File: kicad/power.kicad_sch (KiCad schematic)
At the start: 19 parts, among them J25 ATX-24, J26 External Power, SW2 POWER ON

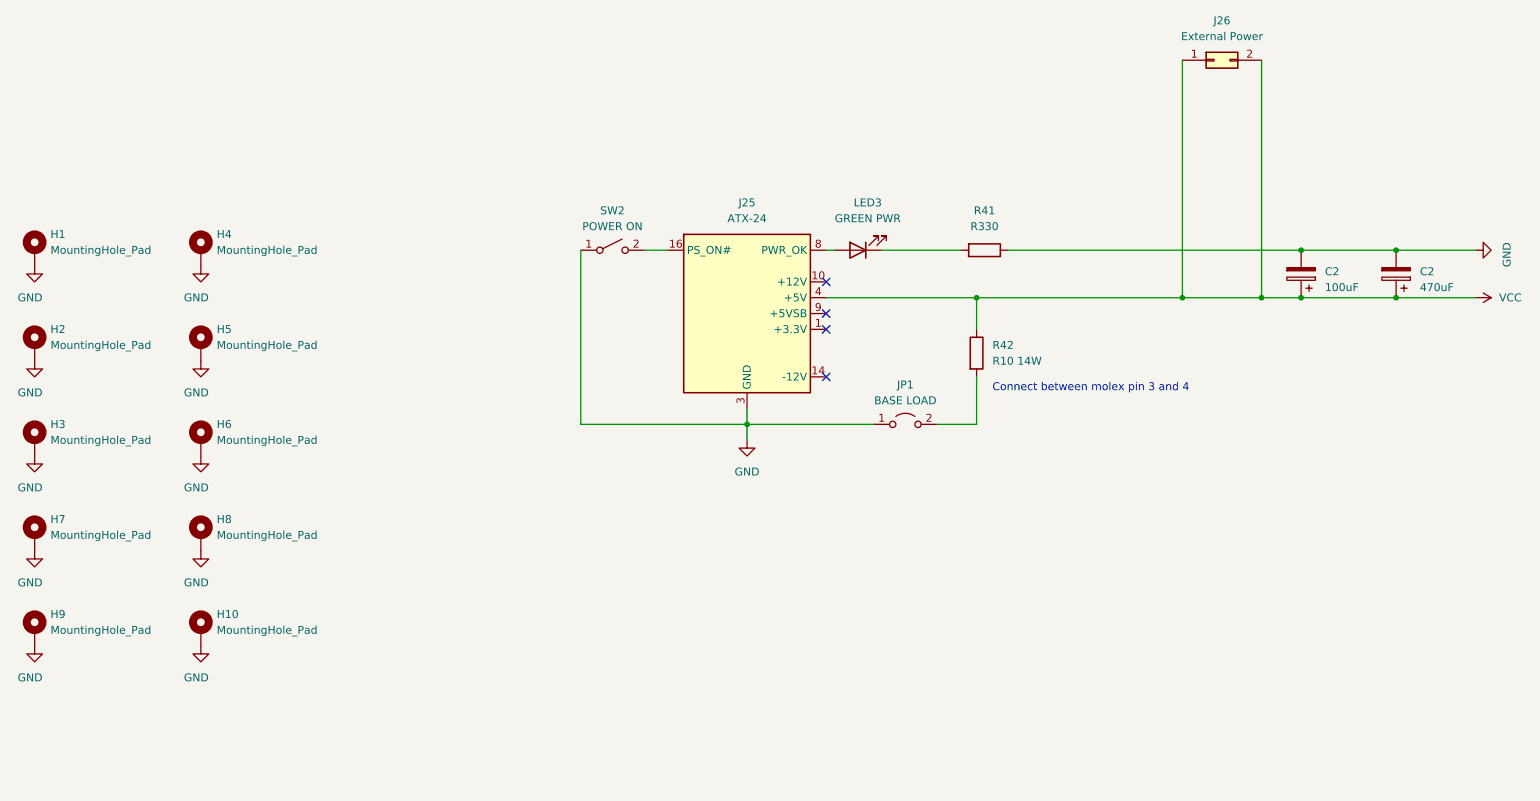
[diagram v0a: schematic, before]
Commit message: fiddlign with placement
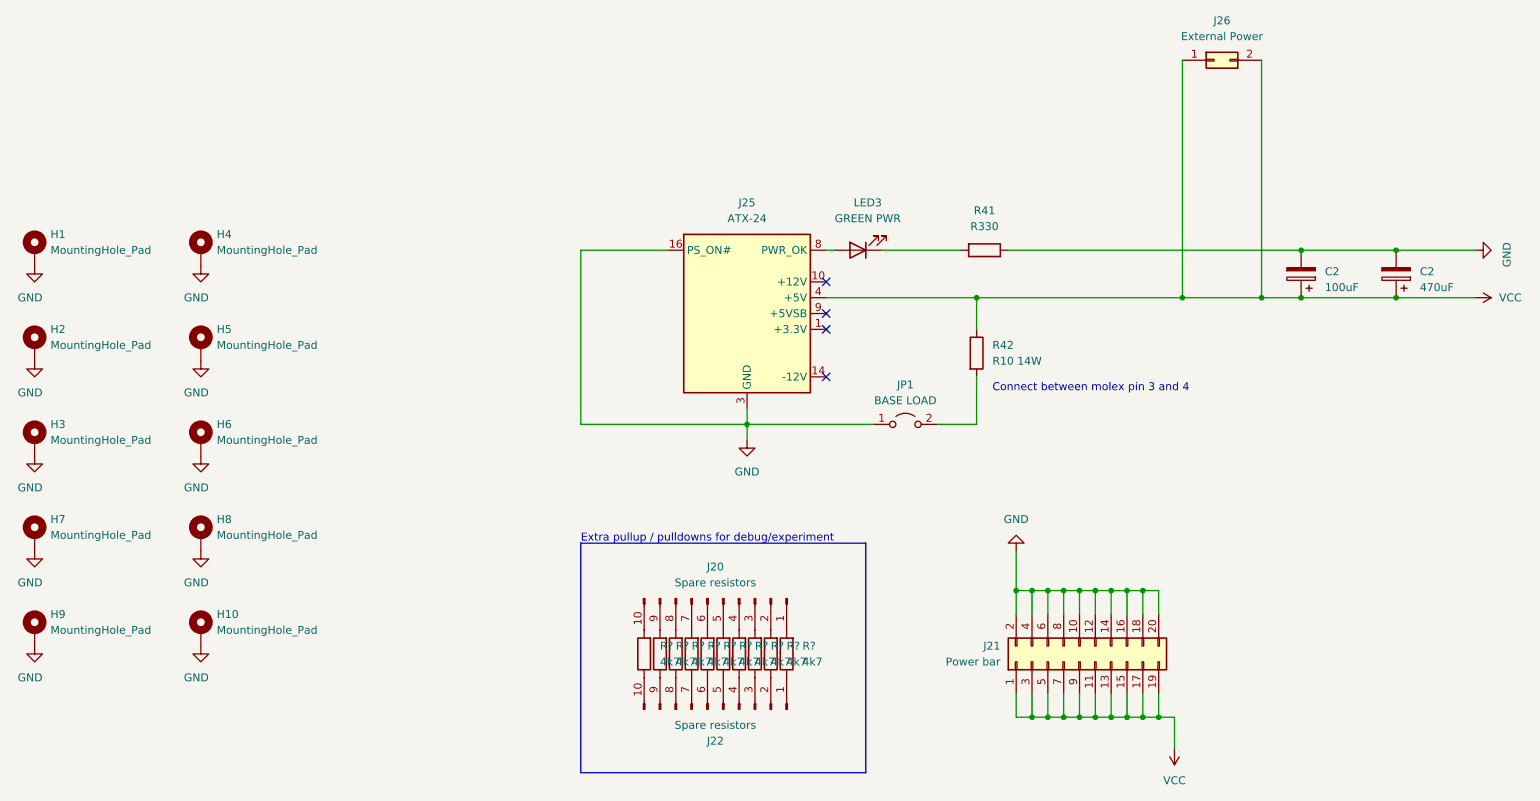
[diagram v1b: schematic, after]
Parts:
- removed SW2: POWER ON, Button_Switch_SMD:SW_DIP_SPSTx01_Slide_6.7x4.1mm_W8.61mm_P2.54mm_LowProfile, symbol Switch:SW_SPST
- added J20, J22: Spare resistors, Connector_PinSocket_2.54mm:PinSocket_1x10_P2.54mm_Vertical, symbol Connector:Conn_01x10_Pin
- added J21: Power bar, Connector_PinSocket_2.54mm:PinSocket_2x10_P2.54mm_Vertical, symbol Connector_Generic:Conn_02x10_Odd_Even
- added R? (x10): 4k7, Resistor_THT:R_Axial_DIN0207_L6.3mm_D2.5mm_P10.16mm_Horizontal, symbol Device:R
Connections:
- net GND: now also J25.16 (PS_ON#), J21.10 (Pin_10), J21.12 (Pin_12), J21.14 (Pin_14), J21.16 (Pin_16), J21.18 (Pin_18), J21.2 (Pin_2), J21.20 (Pin_20), J21.4 (Pin_4), J21.6 (Pin_6), J21.8 (Pin_8)
- net VCC: now also J21.1 (Pin_1), J21.11 (Pin_11), J21.13 (Pin_13), J21.15 (Pin_15), J21.17 (Pin_17), J21.19 (Pin_19), J21.3 (Pin_3), J21.5 (Pin_5), J21.7 (Pin_7), J21.9 (Pin_9)
- new net: J22.10 (Pin_10), R?.1
- new net: J20.10 (Pin_10), R?.2
- new net: J22.3 (Pin_3), R?.1
- new net: J20.3 (Pin_3), R?.2
- new net: J22.7 (Pin_7), R?.1
- new net: J20.7 (Pin_7), R?.2
- new net: J22.1 (Pin_1), R?.1
- new net: J20.1 (Pin_1), R?.2
- new net: J22.8 (Pin_8), R?.1
- new net: J20.8 (Pin_8), R?.2
- new net: J22.2 (Pin_2), R?.1
- new net: J20.2 (Pin_2), R?.2
- new net: J20.4 (Pin_4), R?.2
- new net: J20.5 (Pin_5), R?.2
- new net: J20.6 (Pin_6), R?.2
- new net: J20.9 (Pin_9), R?.2
- new net: J22.4 (Pin_4), R?.1
- new net: J22.5 (Pin_5), R?.1
- new net: J22.6 (Pin_6), R?.1
- new net: J22.9 (Pin_9), R?.1
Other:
- note added: "Extra pullup / pulldowns for debug/experiment"
